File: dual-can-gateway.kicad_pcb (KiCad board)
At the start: 2 copper layers, 101.6 x 88.9 mm, 82 parts, among them J3 Conn_01x02_Pin, Q1 AO3401A, Q2 2N7002, U1 STM32F446RETx, U2 STM32F446RETx, U3 ESP32-WROOM-32UE, U4 TJA1044GT-3, U5 TJA1044GT-3, U6 TJA1055T, U7 TJA1055T, U8 LM2596S-5, U9 AMS1117-3.3

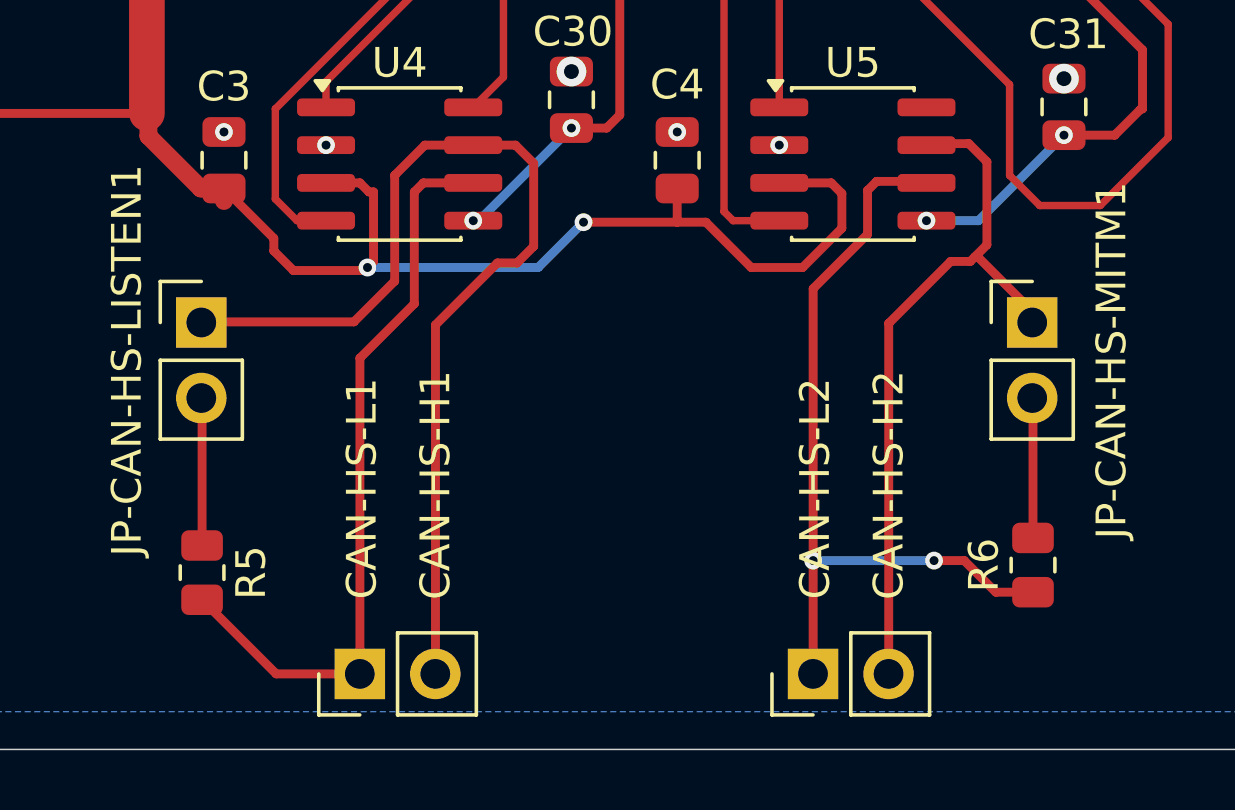
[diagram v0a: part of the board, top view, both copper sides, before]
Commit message: small adjustment
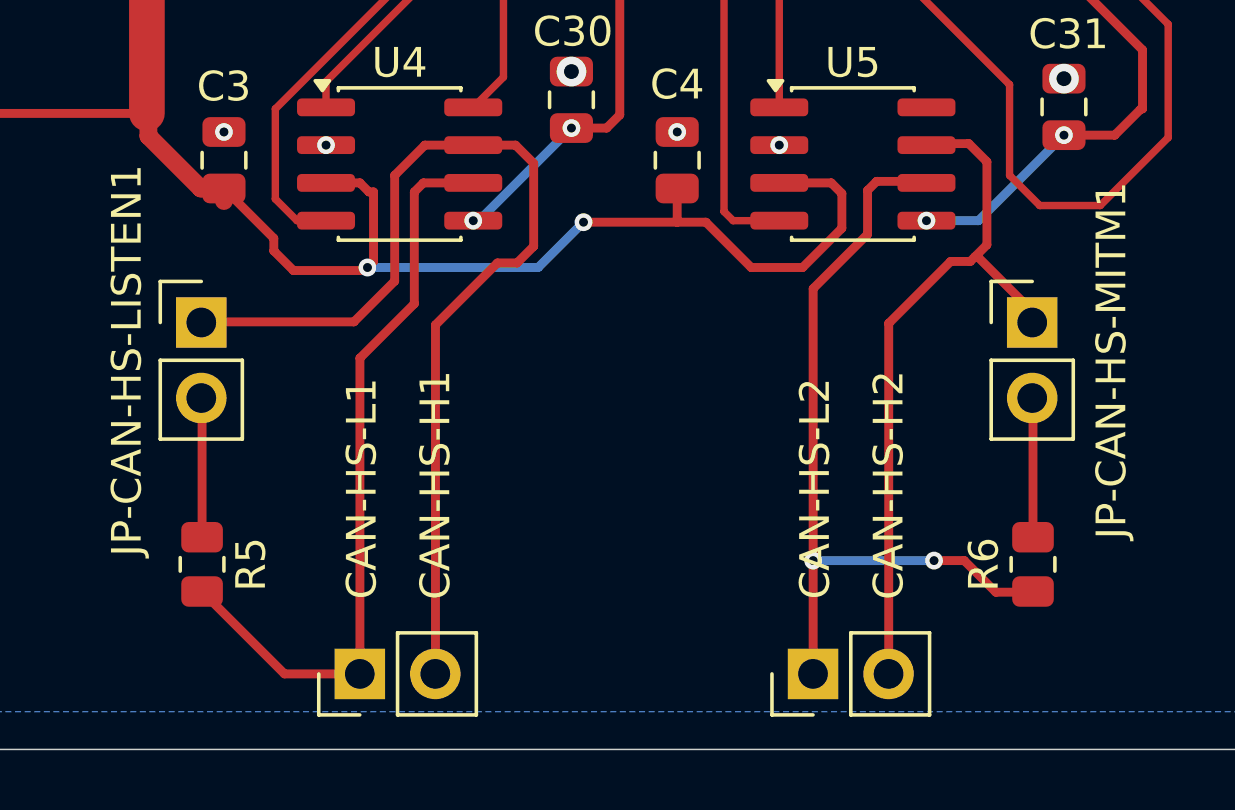
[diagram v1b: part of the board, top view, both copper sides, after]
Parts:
- moved R5 0.28 mm to (63.3, 95.4)
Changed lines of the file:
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@@
 	(footprint "Resistor_SMD:R_0805_2012Metric"
 		(layer "F.Cu")
-		(at 91.212 95.4005 90)
+		(at 91.212 95.377 90)
 		(descr "Resistor SMD 0805 (2012 Metric), square (rectangular) end terminal, IPC-7351 nominal, (Body size source: IPC-SM-782 page 72, https://www.pcb-3d.com/wordpress/wp-content/uploads/ipc-sm-782a_amendment_1_and_2.pdf)")
 		(tags "resistor")
@@
 	(footprint "Resistor_SMD:R_0805_2012Metric"
 		(layer "F.Cu")
-		(at 63.272 95.6545 -90)
+		(at 63.272 95.377 -90)
 		(descr "Resistor SMD 0805 (2012 Metric), square (rectangular) end terminal, IPC-7351 nominal, (Body size source: IPC-SM-782 page 72, https://www.pcb-3d.com/wordpress/wp-content/uploads/ipc-sm-782a_amendment_1_and_2.pdf)")
 		(tags "resistor")
@@
 	)
 	(segment
-		(start 68.58 99.06)
-		(end 65.765 99.06)
+		(start 66.0425 99.06)
+		(end 63.5495 96.567)
 		(width 0.3)
 		(layer "F.Cu")
@@
 	)
 	(segment
-		(start 70.4088 82.8548)
-		(end 70.7136 82.55)
+		(start 68.58 99.06)
+		(end 66.0425 99.06)
 		(width 0.3)
 		(layer "F.Cu")
@@
 	)
 	(segment
-		(start 68.58 88.4428)
-		(end 70.4088 86.614)
+		(start 70.7136 82.55)
+		(end 70.4088 82.8548)
 		(width 0.3)
 		(layer "F.Cu")
@@
 	)
 	(segment
-		(start 68.58 99.06)
-		(end 68.58 88.4428)
+		(start 70.4088 82.8548)
+		(end 70.4088 86.614)
 		(width 0.3)
 		(layer "F.Cu")
@@
 	)
 	(segment
-		(start 70.4088 86.614)
-		(end 70.4088 82.8548)
+		(start 72.39 82.55)
+		(end 70.7136 82.55)
 		(width 0.3)
 		(layer "F.Cu")
@@
 	)
 	(segment
-		(start 65.765 99.06)
-		(end 63.272 96.567)
+		(start 68.58 88.4428)
+		(end 68.58 99.06)
 		(width 0.3)
 		(layer "F.Cu")
@@
 	)
 	(segment
-		(start 70.7136 82.55)
-		(end 72.39 82.55)
+		(start 70.4088 86.614)
+		(end 68.58 88.4428)
 		(width 0.3)
 		(layer "F.Cu")
